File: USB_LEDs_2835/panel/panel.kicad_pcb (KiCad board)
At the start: 2 copper layers, 99.9 x 100 mm, 280 parts, among them U1 MT9284_1, U2 JL8022W-L, U3 74LVC1G04

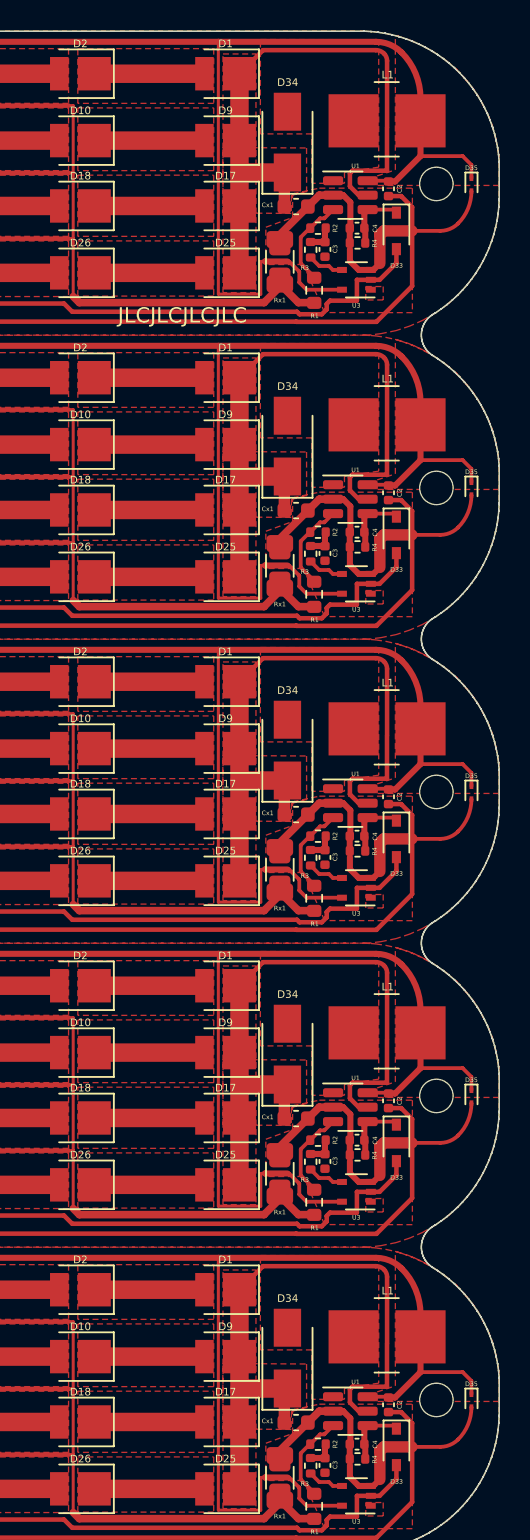
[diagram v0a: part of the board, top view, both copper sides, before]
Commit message: Add files via upload
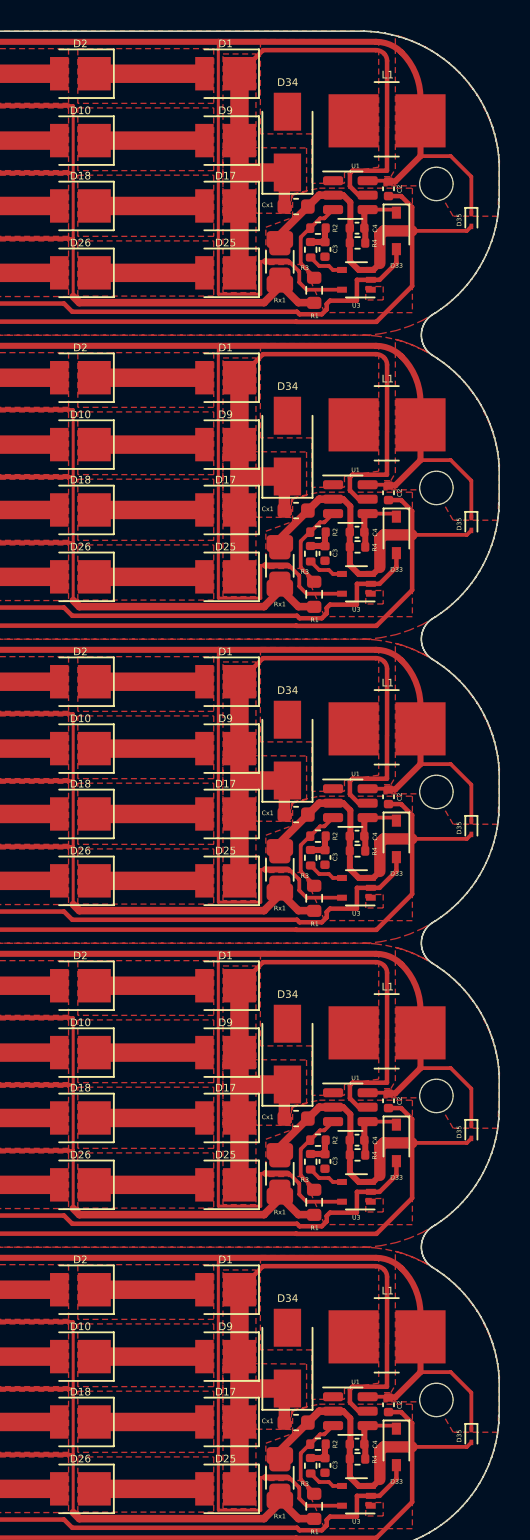
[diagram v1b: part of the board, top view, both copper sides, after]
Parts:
- removed the D35 at (196.6, 90.1)
- removed the D35 at (196.6, 70.1)
- removed the D35 at (196.6, 110.1)
- removed the D35 at (196.6, 50.1)
- removed the D35 at (196.6, 30.1)
- added D35: D_TVS_unidirection, Diode_SMD:D_SOD-923, F.Cu at (196.6, 52.4)
- added D35: D_TVS_unidirection, Diode_SMD:D_SOD-923, F.Cu at (196.6, 32.4)
- added D35: D_TVS_unidirection, Diode_SMD:D_SOD-923, F.Cu at (196.6, 92.4)
- added D35: D_TVS_unidirection, Diode_SMD:D_SOD-923, F.Cu at (196.6, 72.4)
- added D35: D_TVS_unidirection, Diode_SMD:D_SOD-923, F.Cu at (196.6, 112.4)
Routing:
- net Board_4-+5V: track 149.2 -> 151.0 mm
- net Board_3-+5V: track 149.2 -> 151.0 mm
- net Board_2-+5V: track 149.2 -> 151.0 mm
- net Board_0-+5V: track 149.2 -> 151.0 mm
- net Board_1-+5V: track 149.2 -> 151.0 mm
- net Board_2-GND: track 162.3 -> 160.8 mm
- net Board_0-GND: track 162.3 -> 160.8 mm
- net Board_1-GND: track 162.3 -> 160.8 mm
- net Board_4-GND: track 162.3 -> 160.8 mm
- net Board_3-GND: track 162.3 -> 160.8 mm
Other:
- board text removed: "JLCJLCJLCJLC"
